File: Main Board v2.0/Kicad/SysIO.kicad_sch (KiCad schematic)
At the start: 8 parts, among them J10 SPI, J6 AVR-JTAG-10, J7 USART0, J8 USART1, J9 PS2KB, U10 ATmega1284-P, U11 74HCT245, Y2 32.768kHz

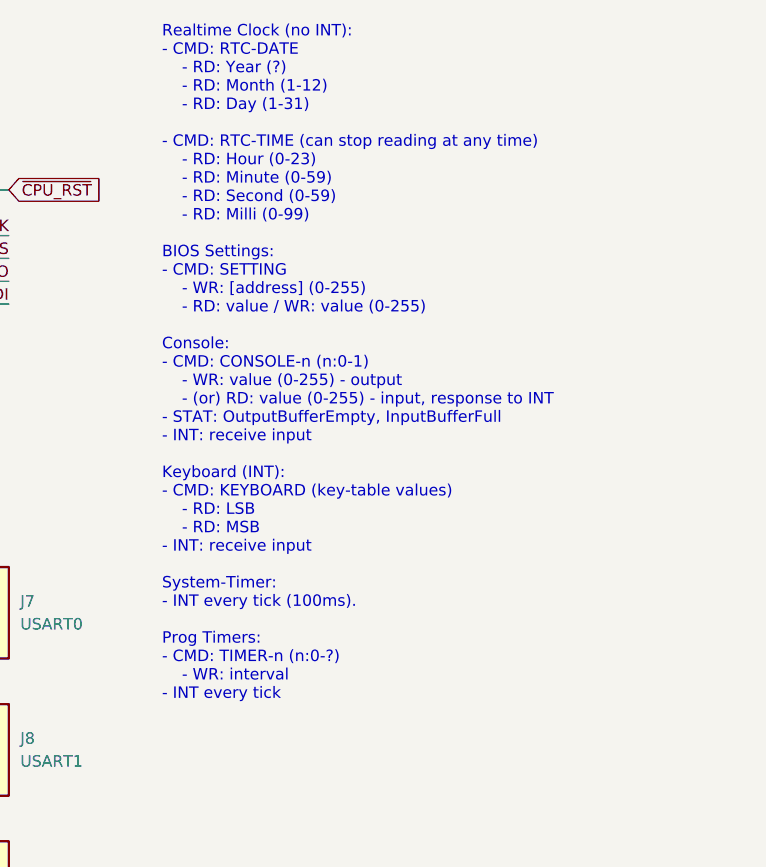
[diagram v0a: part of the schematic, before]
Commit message: docs
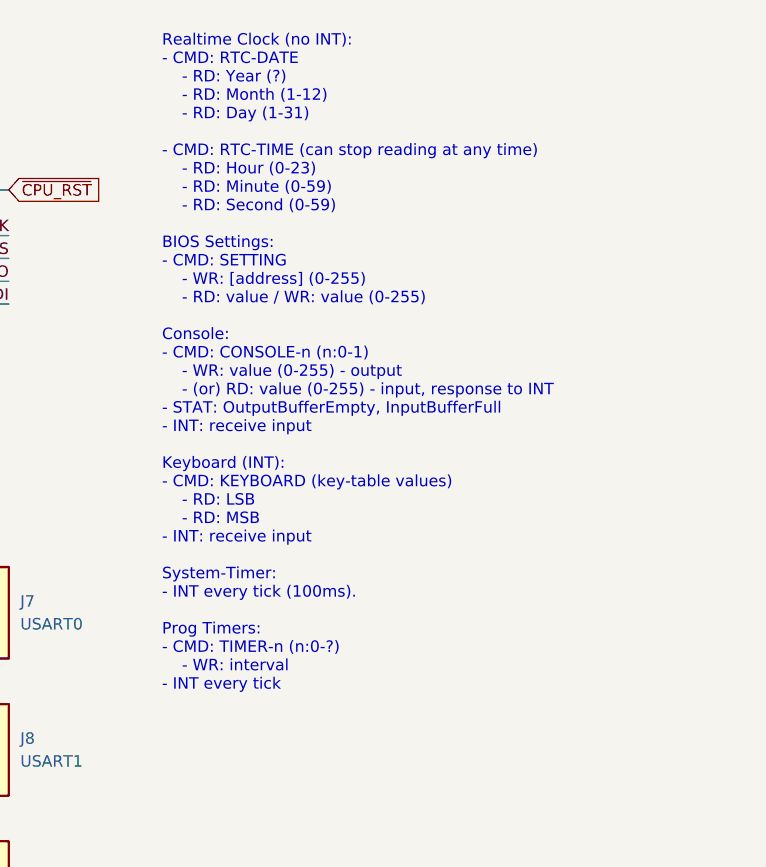
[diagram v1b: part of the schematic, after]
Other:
- note added: "Realtime Clock (no INT): - CMD: RTC-DATE - RD: Year (?) - RD: Month (1-12) - RD: Day (1-31) - CMD: RTC-TIME (can stop reading at any time) - RD: Hour (0-23) - RD: Minute (0-59) - RD: Second (0-59) BIOS Settings: - CMD: SETTING - WR: [address] (0-255) - RD: value / WR: value (0-255) Console: - CMD: CONSOLE-n (n:0-1) - WR: value (0-255) - output - (or) RD: value (0-255) - input, response to INT - S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"
- note removed: "Realtime Clock (no INT): - CMD: RTC-DATE - RD: Year (?) - RD: Month (1-12) - RD: Day (1-31) - CMD: RTC-TIME (can stop reading at any time) - RD: Hour (0-23) - RD: Minute (0-59) - RD: Second (0-59) - RD: Milli (0-99) BIOS Settings: - CMD: SETTING - WR: [address] (0-255) - RD: value / WR: value (0-255) Console: - CMD: CONSOLE-n (n:0-1) - WR: value (0-255) - output - (or) RD: value (0-255) - input, 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"
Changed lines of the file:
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@@
 		)
 	)
-	(text "Realtime Clock (no INT):\n- CMD: RTC-DATE\n	- RD: Year (?)\n	- RD: Month (1-12)\n	- RD: Day (1-31)\n\n- CMD: RTC-TIME (can stop reading at any time)\n	- RD: Hour (0-23)\n	- RD: Minute (0-59)\n	- RD: Second (0-59)\n	- RD: Milli (0-99)\n\nBIOS Settings:\n- CMD: SETTING\n	- WR: [address] (0-255)\n	- RD: value / WR: value (0-255)\n\nConsole:\n- CMD: CONSOLE-n (n:0-1)\n	- WR: value (0-255) - output\n	- (or) RD: value (0-255) - input, response to INT\n- STAT: OutputBufferEmpty, InputBufferFull\n- INT: receive input\n\nKeyboard (INT):\n- CMD: KEYBOARD (key-table values)\n	- RD: LSB\n	- RD: MSB\n- INT: receive input\n\nSystem-Timer:\n- INT every tick (100ms).\n\nProg Timers:\n- CMD: TIMER-n (n:0-?)\n	- WR: interval\n- INT every tick\n"
+	(text "Realtime Clock (no INT):\n- CMD: RTC-DATE\n	- RD: Year (?)\n	- RD: Month (1-12)\n	- RD: Day (1-31)\n\n- CMD: RTC-TIME (can stop reading at any time)\n	- RD: Hour (0-23)\n	- RD: Minute (0-59)\n	- RD: Second (0-59)\n\nBIOS Settings:\n- CMD: SETTING\n	- WR: [address] (0-255)\n	- RD: value / WR: value (0-255)\n\nConsole:\n- CMD: CONSOLE-n (n:0-1)\n	- WR: value (0-255) - output\n	- (or) RD: value (0-255) - input, response to INT\n- STAT: OutputBufferEmpty, InputBufferFull\n- INT: receive input\n\nKeyboard (INT):\n- CMD: KEYBOARD (key-table values)\n	- RD: LSB\n	- RD: MSB\n- INT: receive input\n\nSystem-Timer:\n- INT every tick (100ms).\n\nProg Timers:\n- CMD: TIMER-n (n:0-?)\n	- WR: interval\n- INT every tick\n"
 		(exclude_from_sim no)
 		(at 224.028 58.674 0)
